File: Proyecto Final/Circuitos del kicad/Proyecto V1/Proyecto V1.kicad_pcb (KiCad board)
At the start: 2 copper layers, 14 parts, among them J1 12v, J2 I2C + LCD, J3 DS1307, SW1 SW_Push, SW2 SW_Push, SW3 SW_Push, SW4 SW_Push, U1 LM7805_TO220, U2 DS18B20, U3 ATmega328P-P

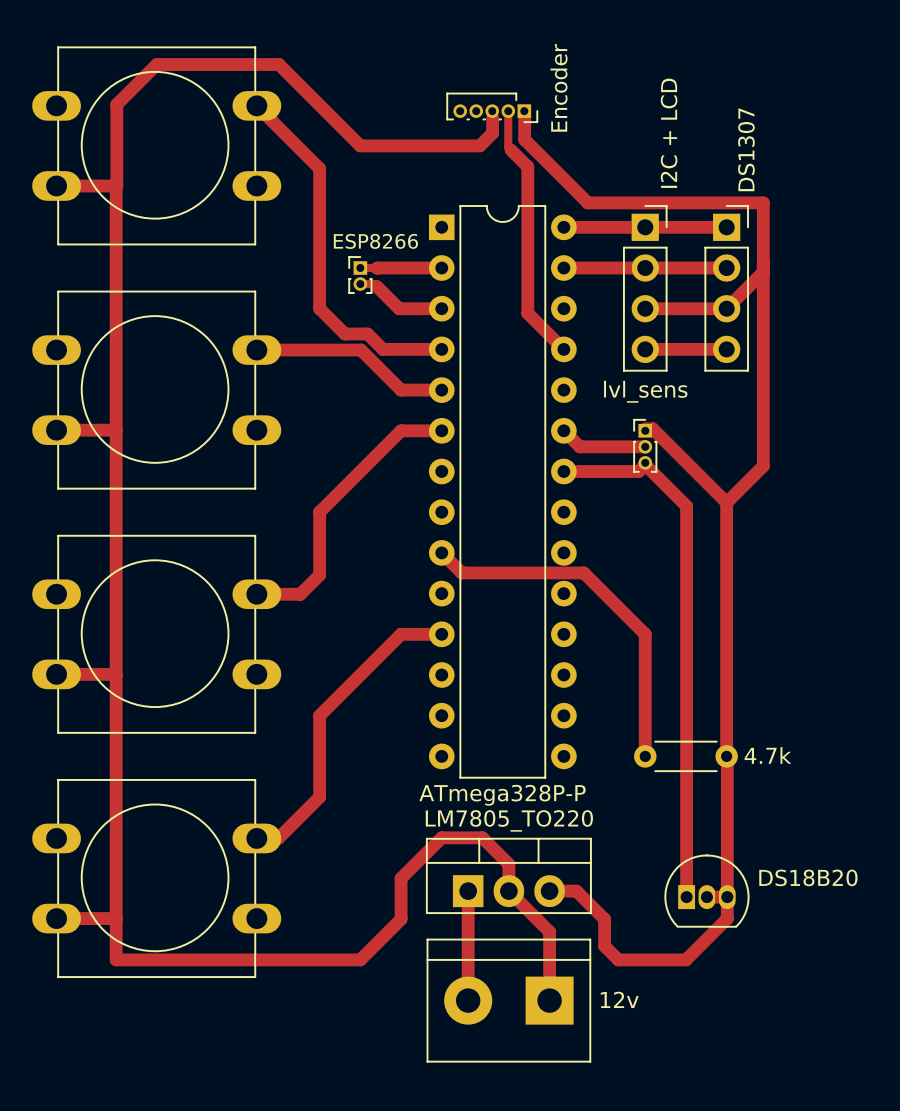
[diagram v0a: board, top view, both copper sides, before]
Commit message: save kicad
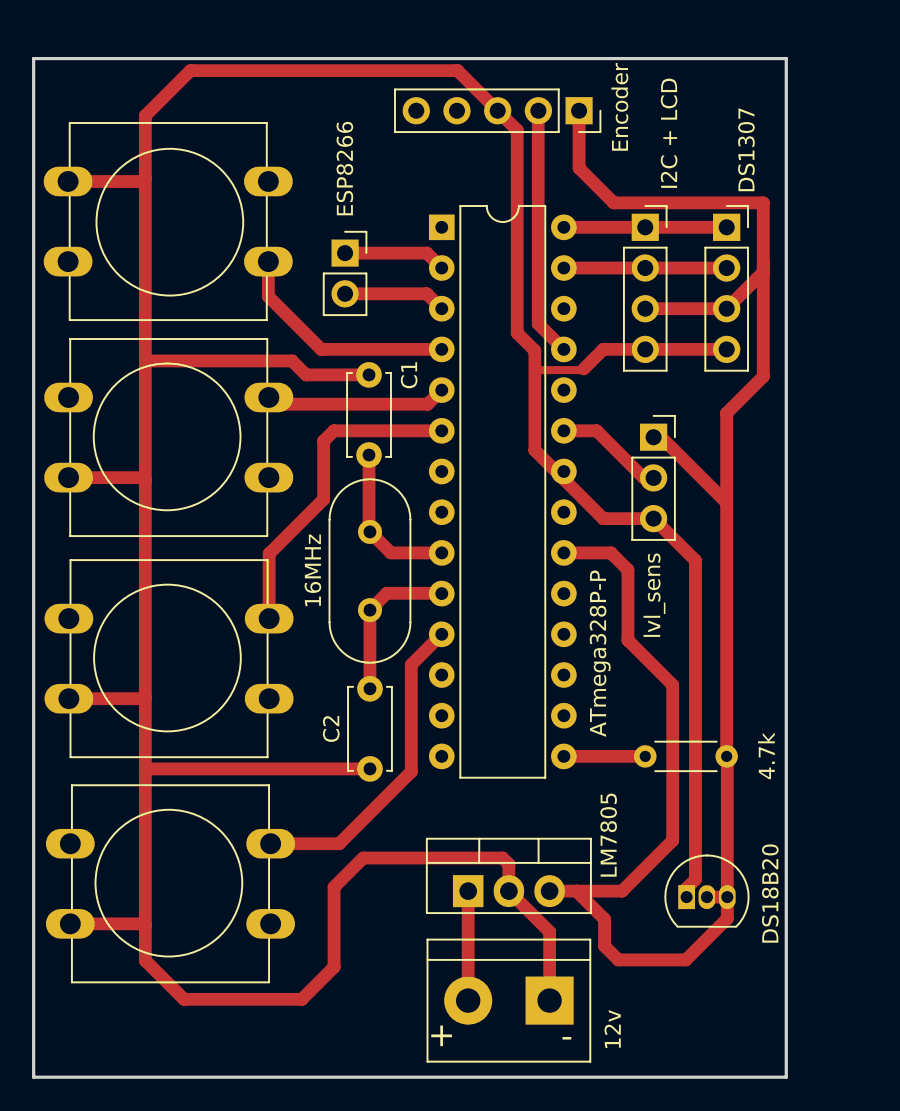
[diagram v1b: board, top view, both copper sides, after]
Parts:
- added C1: 20pF, Capacitor_THT:C_Disc_D5.0mm_W2.5mm_P5.00mm, F.Cu at (152.9, 70.1)
- added C2: 20pF, Capacitor_THT:C_Disc_D5.0mm_W2.5mm_P5.00mm, F.Cu at (153.0, 84.7)
- added Y1: 16MHz, Crystal:Crystal_HC49-4H_Vertical, F.Cu at (153.0, 74.9)
- Lvl_sens1: renamed from --------1; footprint Connector_PinHeader_1.00mm:PinHeader_1x03_P1.00mm_Vertical -> Connector_PinSocket_2.54mm:PinSocket_1x03_P2.54mm_Vertical
- RV1: footprint Connector_PinSocket_1.00mm:PinSocket_1x05_P1.00mm_Vertical -> Connector_PinSocket_2.54mm:PinSocket_1x05_P2.54mm_Vertical
- U1: value LM7805_TO220 -> LM7805
- s1: footprint Connector_PinHeader_1.00mm:PinHeader_1x02_P1.00mm_Vertical -> Connector_PinSocket_2.54mm:PinSocket_1x02_P2.54mm_Vertical
- moved SW1 11.8 mm to (134.2, 53.0), turned to 0 degrees
- moved RV1 3.42 mm to (166.1, 48.6)
- moved SW2 3.05 mm to (146.7, 71.5)
- moved SW3 1.70 mm to (146.7, 85.3)
- moved s1 1.33 mm to (151.4, 57.5)
- moved SW4 0.92 mm to (146.8, 99.3)
- moved Lvl_sens1 0.66 mm to (170.7, 69.0)
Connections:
- R1 pad 2: Net-(R1-Pad2) -> Net-(U3-Pad15)
- U3 pad 10: unconnected-(U3-Pad10) -> Net-(C2-Pad1)
- U3 pad 15: unconnected-(U3-Pad15) -> Net-(U3-Pad15)
- U3 pad 9: Net-(R1-Pad2) -> Net-(C1-Pad1)
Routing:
- net GND: track 174.2 -> 233.5 mm
- net +5V: track 96.6 -> 123.3 mm
- net Net-(R1-Pad2): track 22.4 -> 0.00 mm
- net Net-(C1-Pad1): track 0.00 -> 10.1 mm
- net Net-(C2-Pad1): track 0.00 -> 9.83 mm
- net Net-(SW1-Pad2): track 23.0 -> 14.4 mm
- net Net-(U3-Pad15): track 0.00 -> 5.08 mm
- net Net-(SW3-Pad2): track 18.1 -> 20.1 mm
- net Net-(U3-Pad2): track 5.09 -> 6.42 mm
- net Net-(U3-Pad23): track 5.49 -> 6.82 mm
- net Net-(SW2-Pad2): track 12.6 -> 11.3 mm
- net Net-(RV1-Pad2): track 16.3 -> 15.6 mm
- net Net-(U3-Pad3): track 5.72 -> 6.42 mm
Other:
- board outline added: 47 x 63.6 mm
- board text added: "+"
- board text added: "-"
